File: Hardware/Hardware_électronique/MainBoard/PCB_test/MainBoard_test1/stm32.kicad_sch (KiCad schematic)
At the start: 83 parts, among them J2 Conn_ST_STDC14, J3 USB_A, SW1 SW_Push, SW2 SW_Push, SW3 SW_Push, SW4 SW_Push, U1 STM32H735IGTx, U4 AZ1117-3.3

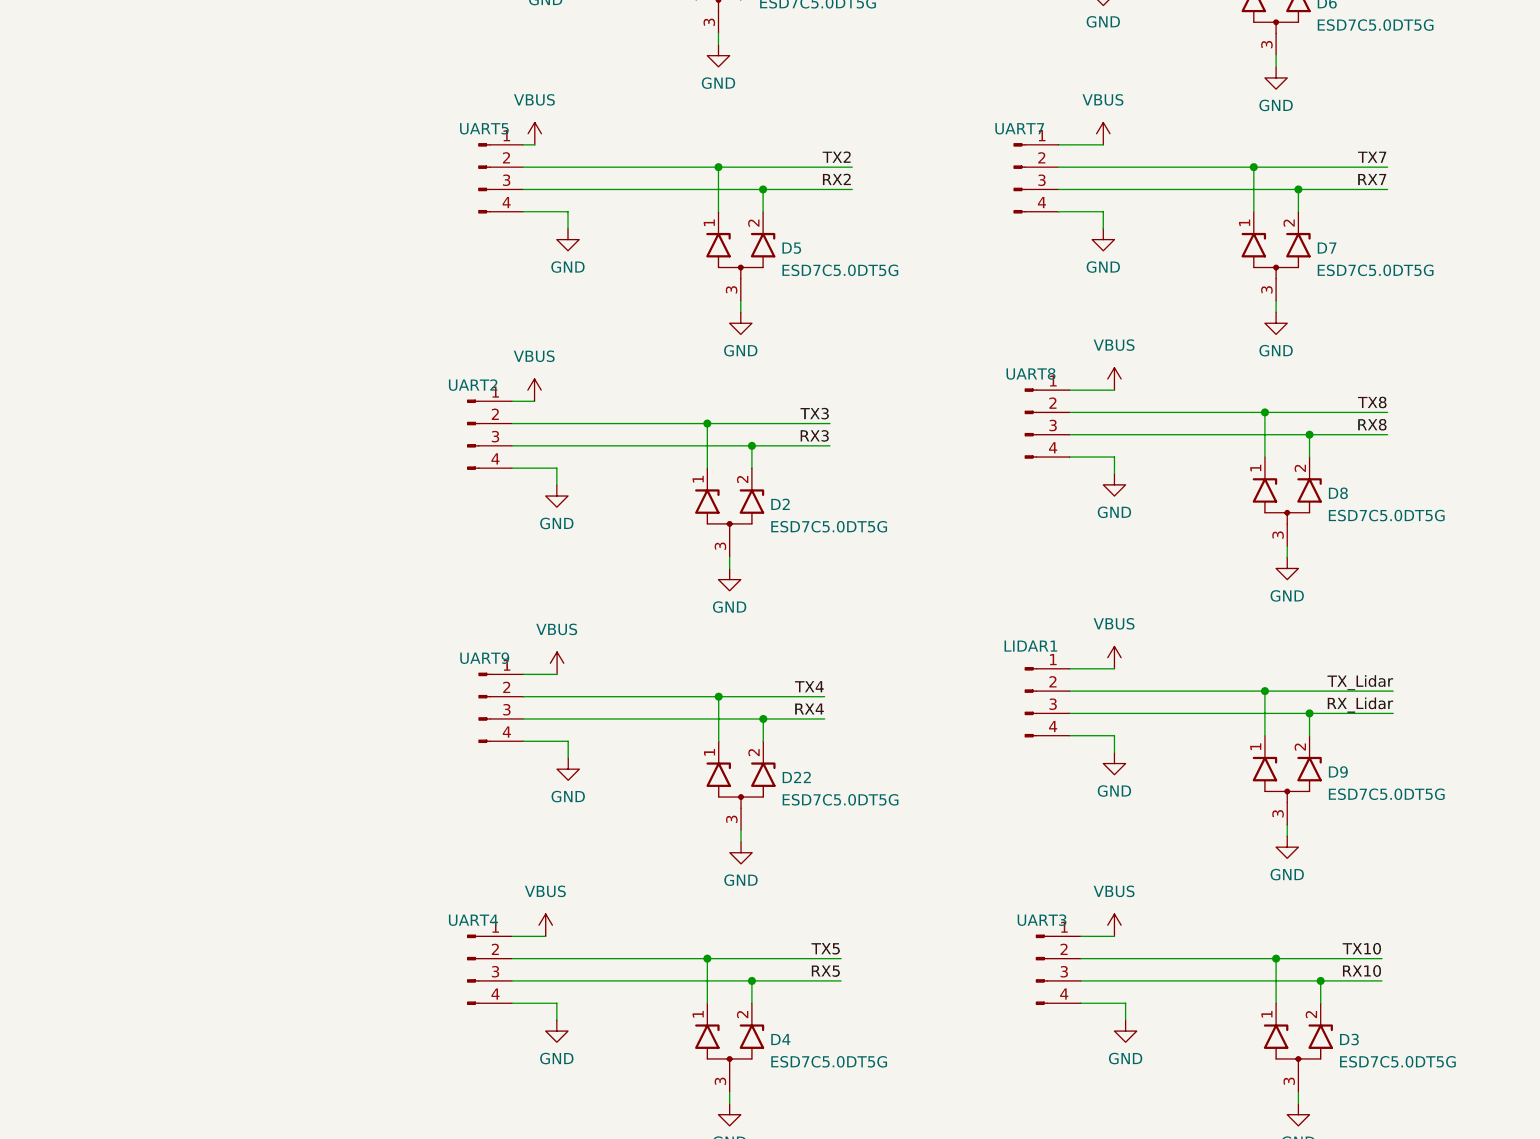
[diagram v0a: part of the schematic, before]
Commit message: quite finished schematics
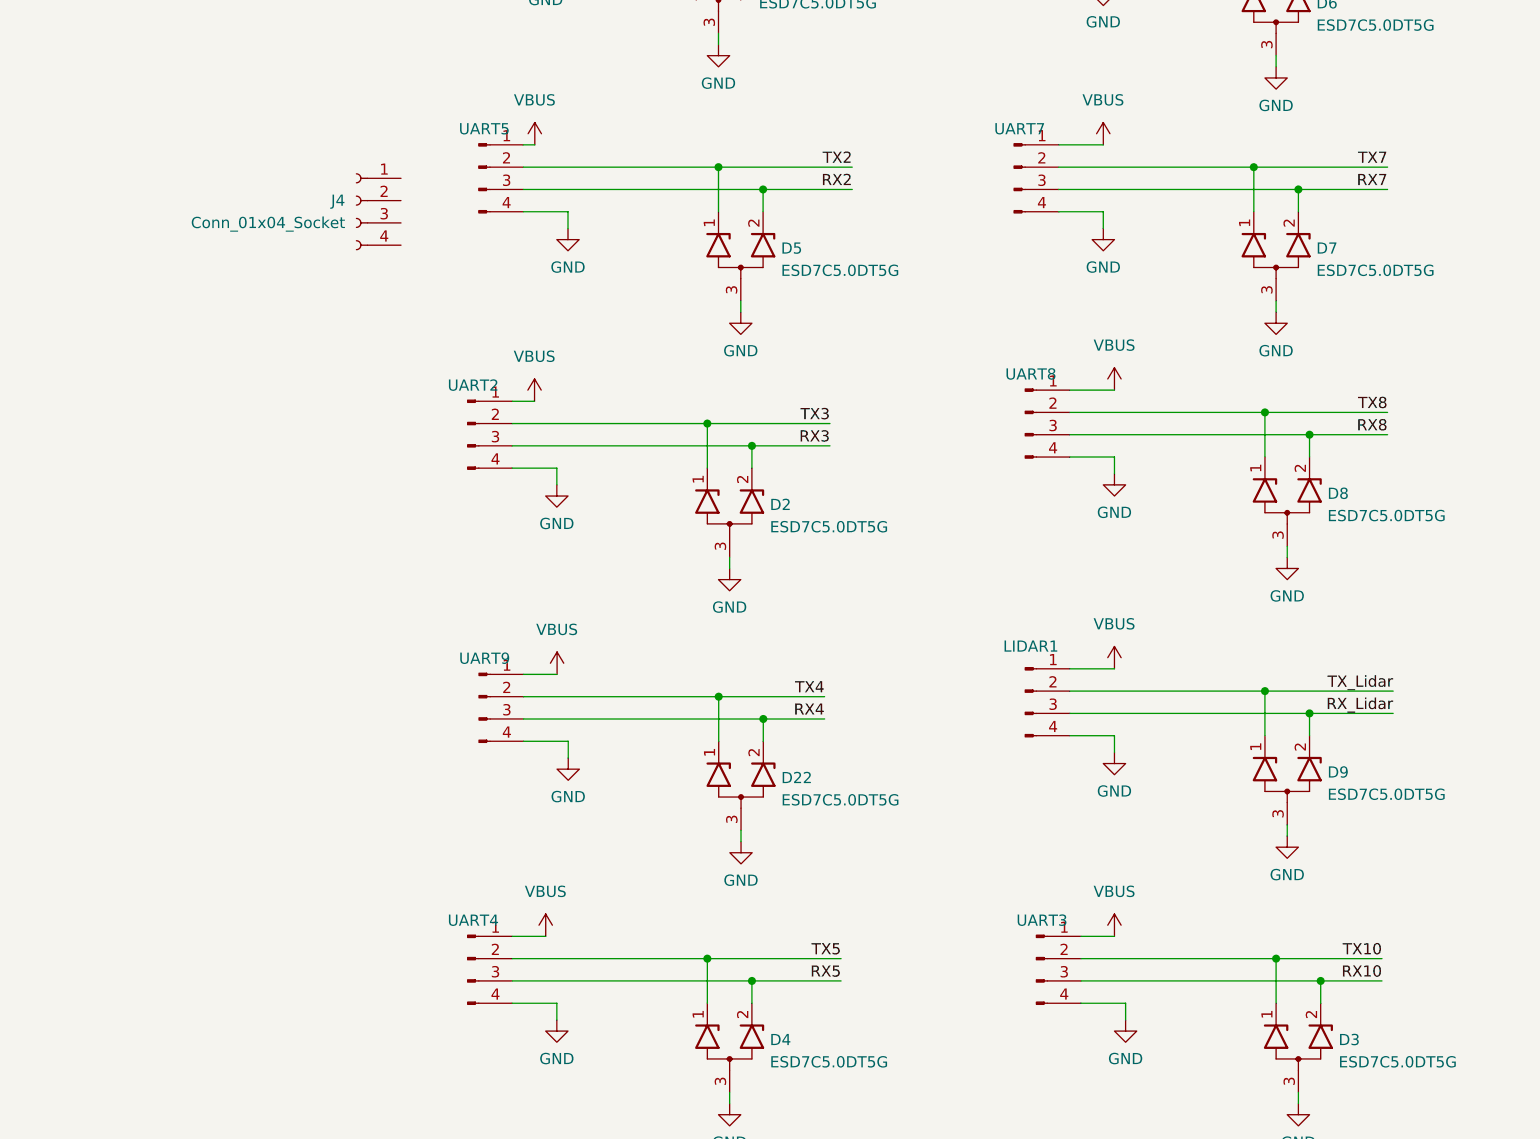
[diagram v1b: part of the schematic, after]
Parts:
- added J4: Conn_01x04_Socket, Connector_JST:JST_XH_B4B-XH-A_1x04_P2.50mm_Vertical, symbol Connector:Conn_01x04_Socket
